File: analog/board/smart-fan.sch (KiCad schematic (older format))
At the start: 34 parts, among them J1 TEMP_In, J2 12V_PWR, J3 12V_In, J4 FAN_Out, J5 FAN_Out, J6 FAN_Out, Q1 BC817, Q2 Q_PMOS_GSD, Q3 Q_PMOS_GSD, Q4 BC817, U1 MCP602, U2 AMS1117-5.0, U3 NE555P

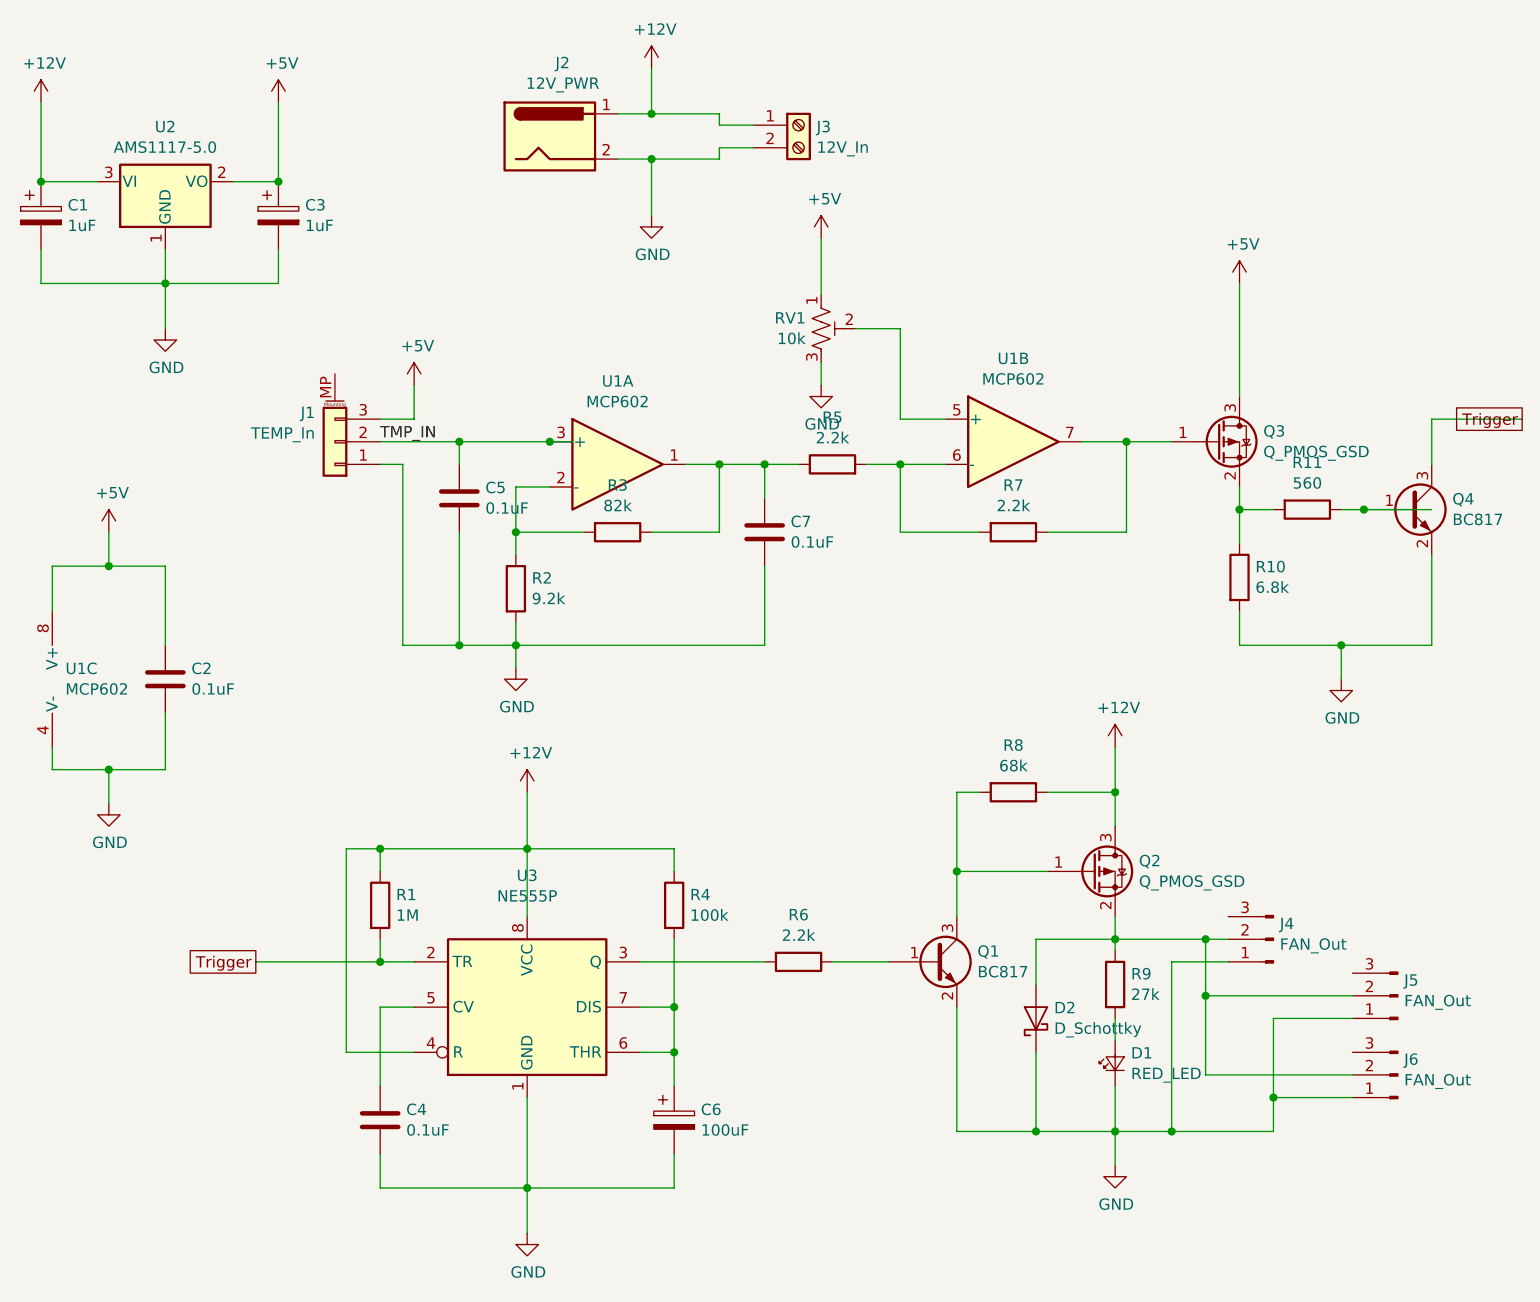
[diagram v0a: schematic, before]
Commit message: WIP: Cleaning up board
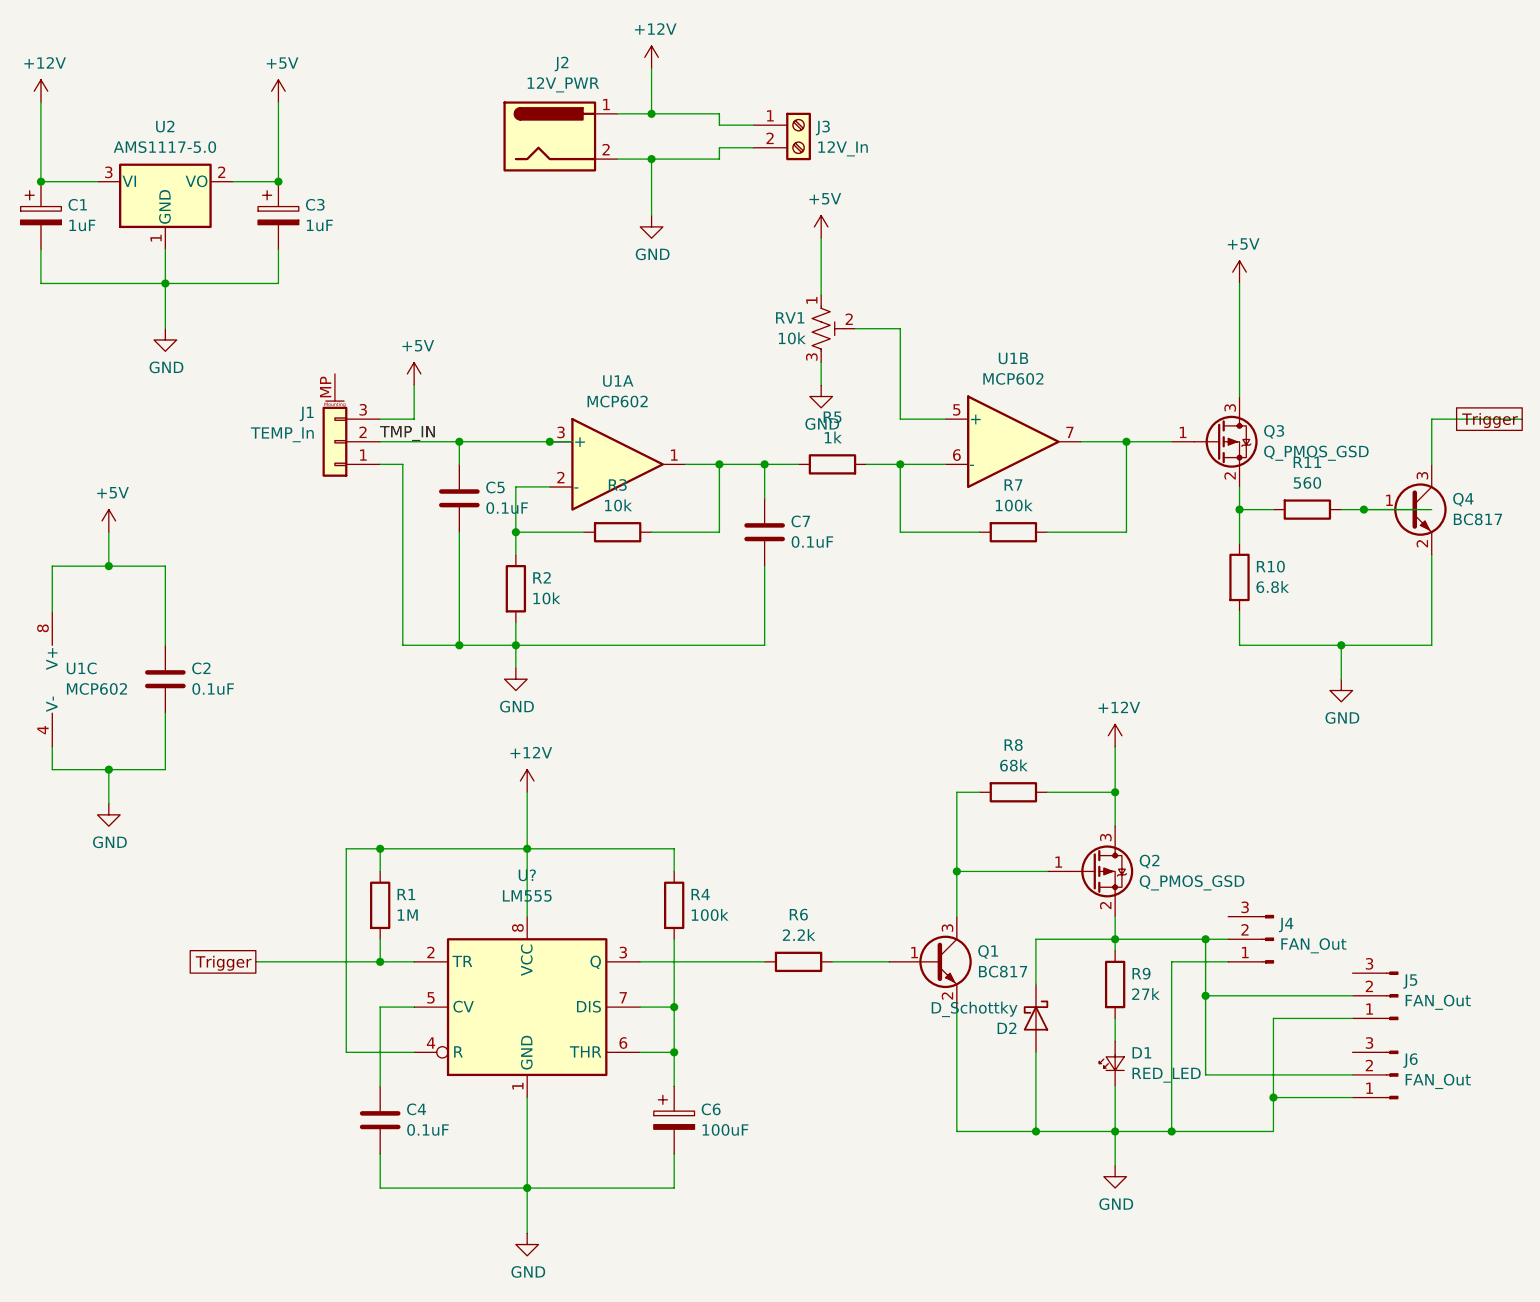
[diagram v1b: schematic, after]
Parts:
- removed U3: NE555P, Package_SO:SOIC-8_5.275x5.275mm_P1.27mm, symbol Timer:NE555P
- added U?: LM555, symbol Timer:LM555
- R2: value 9.2k -> 10k
- R3: value 82k -> 10k
- R5: value 2.2k -> 1k
- R7: value 2.2k -> 100k
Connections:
- net +12V: now also U?.4 (R), U?.8 (VCC)
- net GND: now also D2.2 (A), U?.1 (GND); no longer D2.1 (K)
- net Trigger: now also U?.2 (TR)
- net at J4.2 (Pin_2), J5.2 (Pin_2), J6.2 (Pin_2)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: now also D2.1 (K); no longer D2.2 (A)
- net at R6.2: now also U?.3 (Q)
- net at C4.1: now also U?.5 (CV)
- net at C6.1, R4.2: now also U?.6 (THR), U?.7 (DIS)
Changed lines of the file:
@@
 EELAYER 30 0
 EELAYER END
-$Descr A0 46811 33110
+$Descr A3 16535 11693
 encoding utf-8
 Sheet 1 1
@@
 P 4350 2450
 F 0 "R5" V 4557 2450 50  0000 C CNN
-F 1 "2.2k" V 4466 2450 50  0000 C CNN
+F 1 "1k" V 4466 2450 50  0000 C CNN
 F 2 "Resistor_SMD:R_0805_2012Metric_Pad1.15x1.40mm_HandSolder" V 4280 2450 50  0001 C CNN
 F 3 "~" H 4350 2450 50  0001 C CNN
@@
 P 2950 3000
 F 0 "R2" H 3020 3046 50  0000 L CNN
-F 1 "9.2k" H 3020 2955 50  0000 L CNN
+F 1 "10k" H 3020 2955 50  0000 L CNN
 F 2 "Resistor_SMD:R_0805_2012Metric_Pad1.15x1.40mm_HandSolder" V 2880 3000 50  0001 C CNN
 F 3 "~" H 2950 3000 50  0001 C CNN
@@
 P 3400 2750
 F 0 "R3" V 3193 2750 50  0000 C CNN
-F 1 "82k" V 3284 2750 50  0000 C CNN
+F 1 "10k" V 3284 2750 50  0000 C CNN
 F 2 "Resistor_SMD:R_0805_2012Metric_Pad1.15x1.40mm_HandSolder" V 3330 2750 50  0001 C CNN
 F 3 "~" H 3400 2750 50  0001 C CNN
@@
 P 5150 2750
 F 0 "R7" V 4943 2750 50  0000 C CNN
-F 1 "2.2k" V 5034 2750 50  0000 C CNN
+F 1 "100k" V 5034 2750 50  0000 C CNN
 F 2 "Resistor_SMD:R_0805_2012Metric_Pad1.15x1.40mm_HandSolder" V 5080 2750 50  0001 C CNN
 F 3 "~" H 5150 2750 50  0001 C CNN
@@
 	1150 3800 900  3800
 $Comp
-L Timer:NE555P U3
-U 1 1 5EE81F54
-P 3000 4850
-F 0 "U3" H 3000 5431 50  0000 C CNN
-F 1 "NE555P" H 3000 5340 50  0000 C CNN
-F 2 "Package_SO:SOIC-8_5.275x5.275mm_P1.27mm" H 3650 4450 50  0001 C CNN
-F 3 "http://www.ti.com/lit/ds/symlink/ne555.pdf" H 3850 4450 50  0001 C CNN
-	1    3000 4850
-	1    0    0    -1
-$EndComp
-$Comp
 L smart-fan-rescue:BC817-TransistorBJT Q1
 U 1 1 5EE8608C
@@
 F 3 "~" H 5250 4900 50  0001 C CNN
 	1    5250 4900
-	0    -1   -1   0
+	0    1    1    0
 $EndComp
 Wire Wire Line
@@
 Wire Wire Line
 	5250 5400 5600 5400
+$Comp
+L Timer:LM555 U?
+U 1 1 5F277BFB
+P 3000 4850
+F 0 "U?" H 3000 5431 50  0000 C CNN
+F 1 "LM555" H 3000 5340 50  0000 C CNN
+F 2 "" H 3000 4850 50  0001 C CNN
+F 3 "http://www.ti.com/lit/ds/symlink/lm555.pdf" H 3000 4850 50  0001 C CNN
+	1    3000 4850
+	1    0    0    -1
+$EndComp
 $EndSCHEMATC
